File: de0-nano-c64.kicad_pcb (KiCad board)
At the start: 2 copper layers, 71.6 x 84 mm, 52 parts, among them J1 GPIO_0, J10 SD_Card, J2 PS2_0, J3 PS2_1, J4 AUDIO_L, J5 GPIO_1, J6 VGA_OUT, J7 AUDIO_R, J8 JOYSTICK_1, J9 JOYSTICK_2

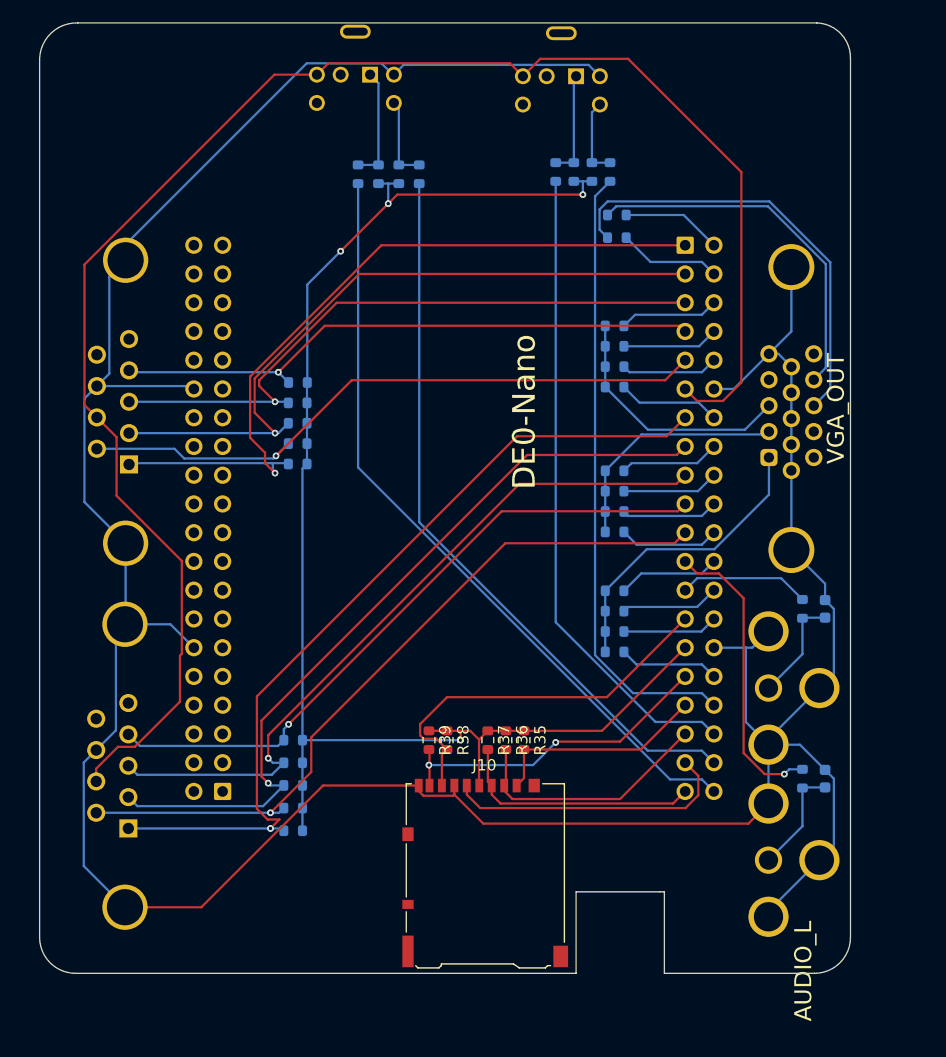
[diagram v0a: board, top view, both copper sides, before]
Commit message: version 1.0
initial version

---------

Co-authored-by: Marek Czerski <m.czerski@ap-tech.pl>
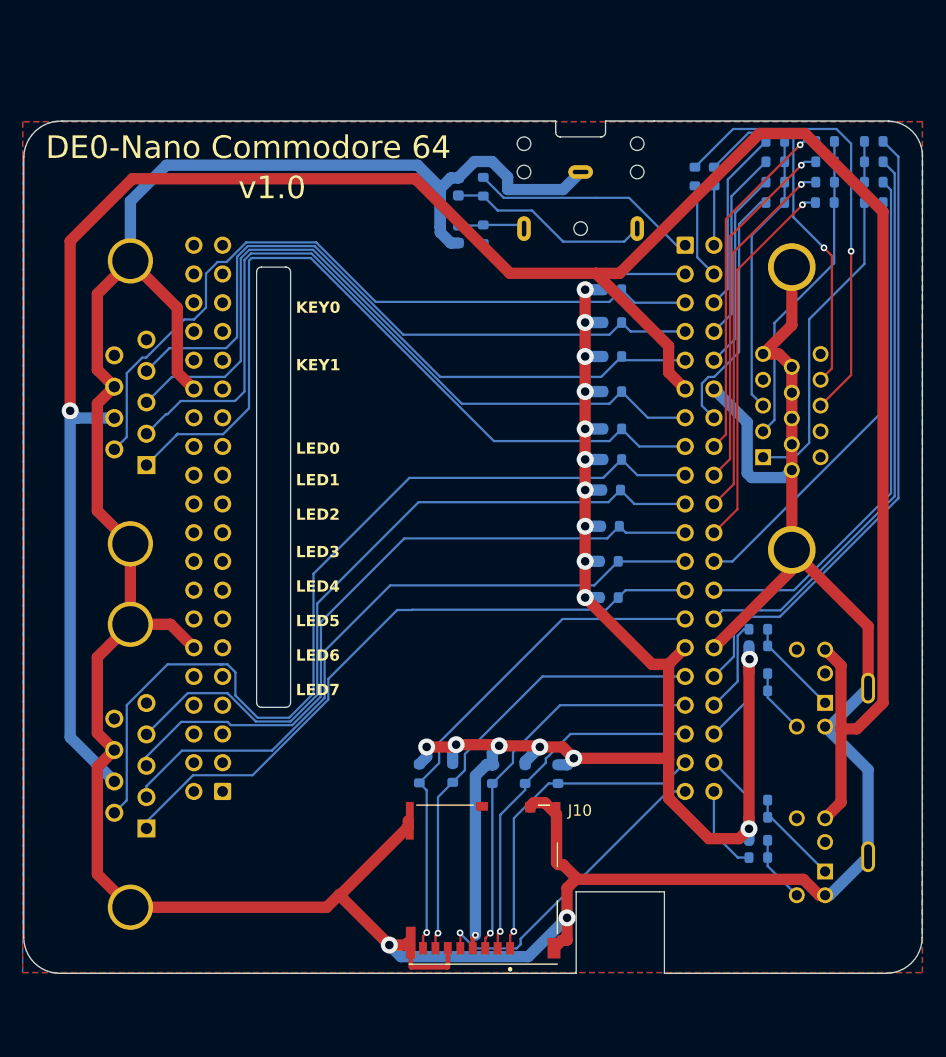
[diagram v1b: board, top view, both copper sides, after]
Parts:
- removed J4: AUDIO_L, 000_LOCAL:RCA
- removed J7: AUDIO_R, 000_LOCAL:RCA
- added J11: AUDIO, 000_LOCAL:Jack_3.5mm_CUI_SJ1-3523N_Horizontal, B.Cu at (154.4, 70.4)
- J10: footprint Connector_Card:microSD_HC_Hirose_DM3AT-SF-PEJM5 -> 000_LOCAL:MOLEX_503398-1892
- J6: value VGA_OUT -> VGA; footprint 000_LOCAL:HD15-SN-25 -> 000_LOCAL:AMPHENOL_ICD15S13E4GV00LF
- J8, J9: footprint Connector_Dsub:DSUB-9_Male_Horizontal_P2.77x2.84mm_EdgePinOffset4.94mm_Housed_MountingHolesOffset7.48mm -> Connector_Dsub:DSUB-9_Male_Horizontal_P2.77x2.84mm_EdgePinOffset7.70mm_Housed_MountingHolesOffset9.12mm
- R35, R36, R37, R38, R39: moved to B.Cu
- moved J3 77.6 mm to (179.8, 130.9), turned to -90 degrees
- moved J2 73.6 mm to (179.8, 116.0), turned to -90 degrees
- moved R19 62.0 mm to (170.1, 130.9), turned to 0 degrees
- moved C1 61.5 mm to (143.6, 71.7)
- moved R21 60.9 mm to (170.1, 129.4), turned to 180 degrees
- moved R22 59.4 mm to (145.8, 71.7)
- moved R20 59.3 mm to (170.1, 127.4), turned to 180 degrees
- moved R18 58.3 mm to (170.1, 125.9), turned to 0 degrees
- moved R17 54.6 mm to (170.1, 116.2), turned to 0 degrees
- moved R15 54.4 mm to (170.1, 114.7), turned to 180 degrees
- moved R16 53.5 mm to (170.1, 110.8), turned to 0 degrees
- moved R14 53.5 mm to (170.1, 112.2), turned to 180 degrees
- moved R13 50.6 mm to (180.3, 67.7)
- moved R1 47.4 mm to (180.3, 69.5)
- moved C2 46.3 mm to (143.6, 75.9), turned to -90 degrees
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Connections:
- J2 pad S1: (no net) -> GND
- J3 pad S1: (no net) -> GND
- J5 pad 1: /J1_UP -> /PWM_L
- J5 pad 13: /J2_UP -> /J1_DOWN
- J5 pad 15: /J2_DOWN -> /J1_UP
- J5 pad 17: /J2_LEFT -> /J2_FIRE
- J5 pad 21: /J2_FIRE -> /J2_LEFT
- J5 pad 23: /PWM_L -> /J2_DOWN
- J5 pad 25: /PWM_R -> /J2_UP
- J5 pad 27: /SD_DAT0 -> /SD_DAT1
- J5 pad 3: /J1_DOWN -> /PWM_R
- J5 pad 31: /SD_DAT1 -> /SD_DAT0
- J5 pad 33: /SD_DAT2 -> /SD_CMD
- J5 pad 34: /PS2_1_CLK -> /PS2_0_DAT
- J5 pad 36: /PS2_1_DAT -> /PS2_0_CLK
- J5 pad 37: /SD_CLK -> /SD_DAT2
- J5 pad 38: /PS2_0_CLK -> /PS2_1_DAT
- J5 pad 39: /SD_CMD -> /SD_CLK
- J5 pad 40: /PS2_0_DAT -> /PS2_1_CLK
- J5 pad 5: /J1_LEFT -> /J1_FIRE
- J5 pad 9: /J1_FIRE -> /J1_LEFT
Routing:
- net +5V: track 148.6 -> 216.7 mm, vias 0 -> 1
- net /PS2_0_DAT: track 68.4 -> 8.24 mm
- net /PS2_0_CLK: track 64.8 -> 5.09 mm
- net /PS2_1_DAT: track 57.0 -> 4.59 mm
- net /R3: track 8.85 -> 56.2 mm
- net /PS2_1_CLK: track 54.7 -> 7.70 mm
- net GND: track 290.6 -> 335.1 mm, vias 0 -> 2
- net /R2: track 8.41 -> 50.4 mm
- net /R1: track 8.72 -> 47.0 mm
- net /R0: track 9.02 -> 38.9 mm
- net /G3: track 8.86 -> 33.4 mm, vias 0 -> 1
- net /G2: track 8.55 -> 32.8 mm, vias 0 -> 1
- net /G1: track 8.54 -> 32.0 mm, vias 0 -> 1
- net /G0: track 8.84 -> 31.3 mm, vias 0 -> 1
- net /J2_UP: track 75.3 -> 57.7 mm, vias 1 -> 0
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- added copper zone on B.Cu, net GND
- added copper zone on F.Cu, net GND
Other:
- board size 71.6 x 84 mm -> 79.4 x 75.3 mm
- board text added: "DE0-Nano Commodore 64"
- board text added: "KEY0"
- board text added: "KEY1"
- board text added: "LED0"
- board text added: "LED1"
- board text added: "LED2"
- board text added: "LED3"
- board text added: "LED4"
- board text added: "LED5"
- board text added: "LED6"
- board text added: "LED7"
- board text added: "v1.0"
- board text removed: "<-USB"
- board text removed: "DAC TRIM"
